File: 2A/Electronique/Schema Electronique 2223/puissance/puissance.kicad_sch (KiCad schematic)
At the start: 45 parts, among them J1 Conn_01x02, J10 Conn_01x02, J11 Conn_01x02, J12 Conn_01x02, J13 Conn_01x02, J14 Conn_01x03, J15 Conn_01x04, J16 Conn_02x20_Counter_Clockwise, J17 Connecteur bouton Arret Urgen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, J18 Bat 2, J19 Bat 1, J2 Conn_01x02, J3 Conn_01x02, J4 Conn_01x02, J5 Conn_01x02, J6 Conn_01x02, J7 Conn_01x02, J8 Conn_01x02, J9 Conn_01x02

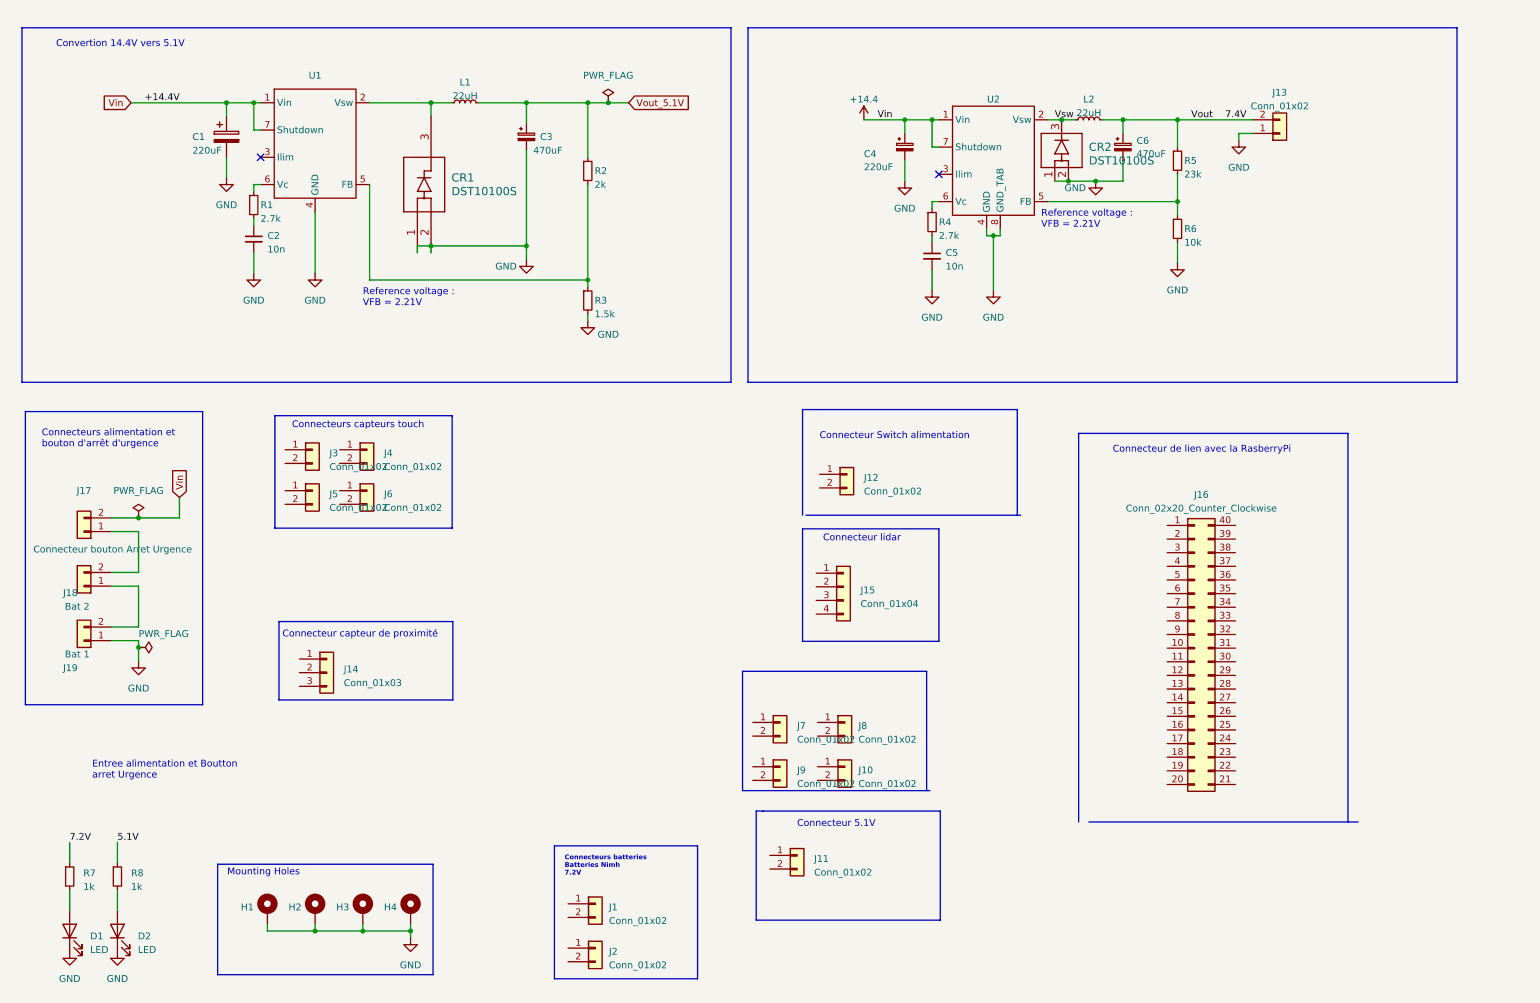
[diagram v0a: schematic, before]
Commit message: update pcb
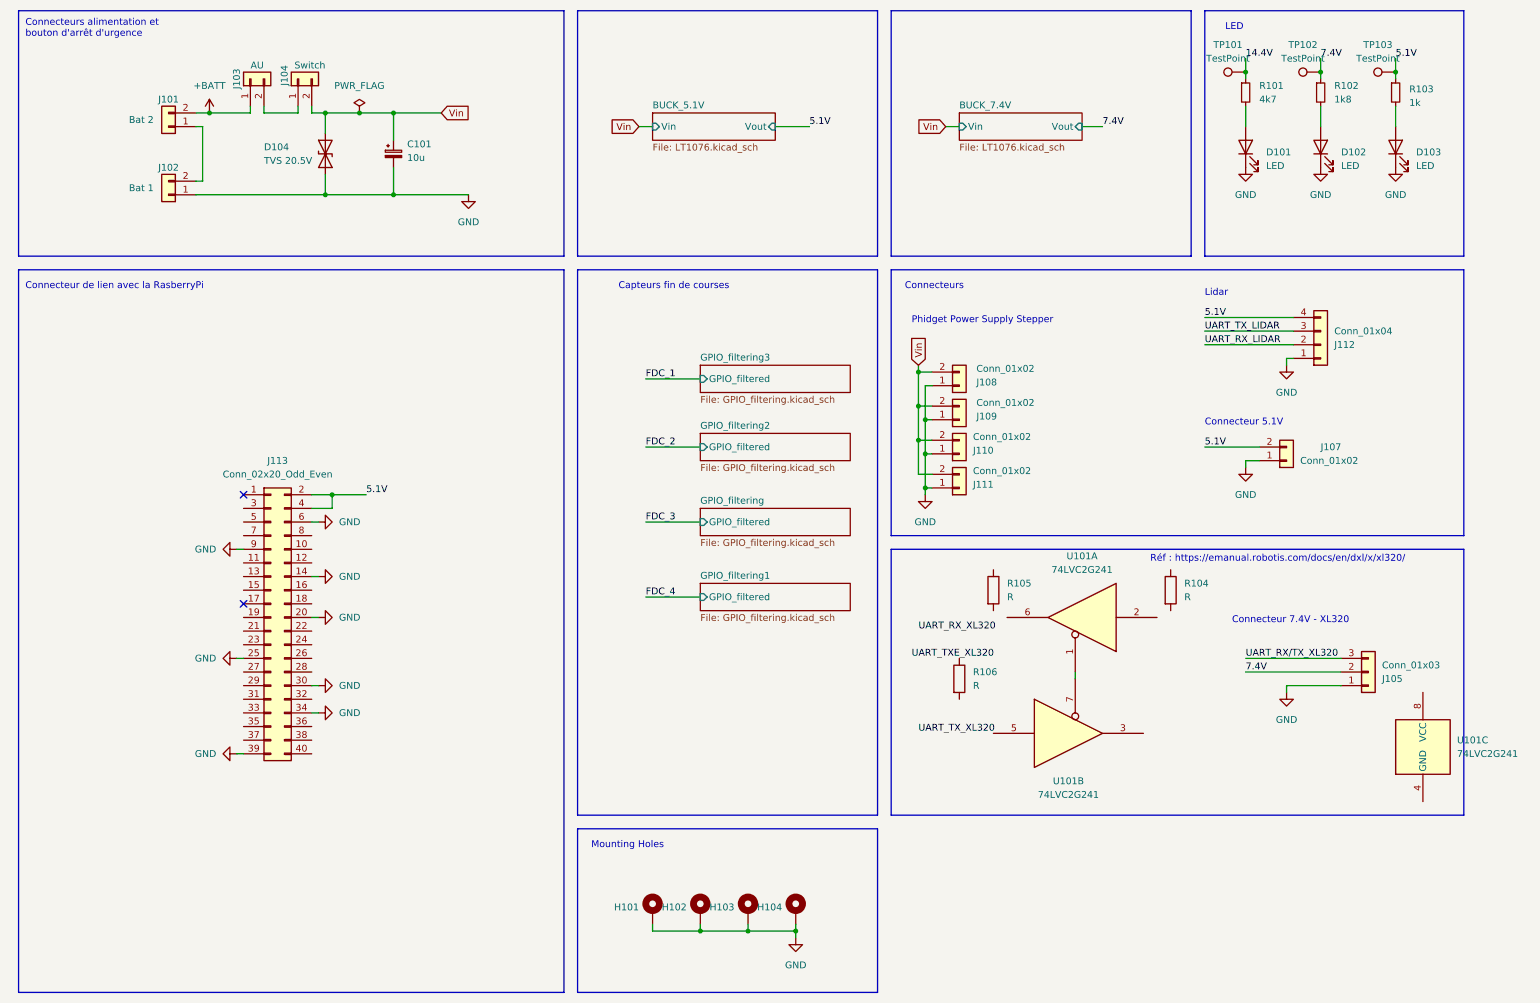
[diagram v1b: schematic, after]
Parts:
- removed C1: 220uF, Capacitor_SMD:C_0603_1608Metric_Pad1.08x0.95mm_HandSolder, symbol Device:C_Polarized
- removed C2, C5: 10n, Capacitor_SMD:C_0603_1608Metric_Pad1.08x0.95mm_HandSolder, symbol Device:C_Small
- removed C3, C6: 470uF, Capacitor_SMD:CP_Elec_10x10.5, symbol Device:C_Polarized_Small
- removed C4: 220uF, Capacitor_SMD:CP_Elec_10x10.5, symbol Device:C_Polarized_Small
- removed CR1: DST10100S, TO277B_LTF, symbol custom:DST10100S
- removed CR2: DST10100S, libs:DST10100S, symbol 2023-03-19_11-33-54:DST10100S
- removed J1, J11, J12, J2, J3, J4, J5, J6: Conn_01x02, symbol Connector_Generic:Conn_01x02
- removed J13: Conn_01x02, Connector_JST:JST_XH_B2B-XH-A_1x02_P2.50mm_Vertical, symbol Connector_Generic:Conn_01x02
- removed J14: Conn_01x03, symbol Connector_Generic:Conn_01x03
- removed J16: Conn_02x20_Counter_Clockwise, symbol Connector_Generic:Conn_02x20_Counter_Clockwise
- removed L1, L2: 22uH, Inductor_SMD:L_Wuerth_WE-PD-Typ-LS_Handsoldering, symbol Device:L_Small
- removed R1, R4: 2.7k, Resistor_SMD:R_0603_1608Metric_Pad0.98x0.95mm_HandSolder, symbol Device:R_Small
- removed R2: 2k, Resistor_SMD:R_0603_1608Metric_Pad0.98x0.95mm_HandSolder, symbol Device:R_Small
- removed R3: 1.5k, Resistor_SMD:R_0603_1608Metric_Pad0.98x0.95mm_HandSolder, symbol Device:R_Small
- removed R5: 23k, Resistor_SMD:R_0603_1608Metric_Pad0.98x0.95mm_HandSolder, symbol Device:R_Small
- removed R6: 10k, Resistor_SMD:R_0603_1608Metric_Pad0.98x0.95mm_HandSolder, symbol Device:R_Small
- removed U1: ~, symbol custom:LT1076
- removed U2: ~, libs:LT1076CR-PBF, symbol custom:LT1076
- added C101: 10u, Capacitor_SMD:CP_Elec_5x5.4, symbol Device:C_Polarized_Small
- added D101: LED, LED_SMD:LED_0603_1608Metric_Pad1.05x0.95mm_HandSolder, symbol Device:LED
- added D104: TVS 20.5V, symbol Diode:1.5KExxCA
- added J104: Switch, symbol Connector_Generic:Conn_01x02
- added J105: Conn_01x03, symbol Connector_Generic:Conn_01x03
- added J107: Conn_01x02, symbol Connector_Generic:Conn_01x02
- added J113: Conn_02x20_Odd_Even, symbol Connector_Generic:Conn_02x20_Odd_Even
- added R101: 4k7, Resistor_SMD:R_0603_1608Metric_Pad0.98x0.95mm_HandSolder, symbol Device:R_Small
- added R104, R105, R106: R, symbol Device:R
- added TP101, TP102, TP103: TestPoint, symbol Connector:TestPoint
- added U101: 74LVC2G241, symbol 74xGxx:74LVC2G241
- J103: renamed from J17; value Connecteur bouton Arret Urgence -> AU
- R102: renamed from R7; value 1k -> 1k8
- renumbered D1 to D102, D2 to D103, H1 to H101, H2 to H102, H3 to H103, H4 to H104, J18 to J101, J19 to J102, J9 to J108, J7 to J109, J8 to J110, J10 to J111, J15 to J112, R8 to R103
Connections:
- net 7.2V is gone; now on net 7.4V: R102.1
- net 5.1V: now also J112.4 (Pin_4), J107.2 (Pin_2), J113.2 (Pin_2), J113.4 (Pin_4), TP103.1
- net 7.4V: now also J105.2 (Pin_2), TP102.1
- net GND: now also J108.1 (Pin_1), J109.1 (Pin_1), J110.1 (Pin_1), J111.1 (Pin_1), J112.1 (Pin_1), C101.2, D101.1 (K), D104.2 (A2), J105.1 (Pin_1), J107.1 (Pin_1), J113.14 (Pin_14), J113.20 (Pin_20), J113.25 (Pin_25), J113.30 (Pin_30), J113.34 (Pin_34), J113.39 (Pin_39), J113.6 (Pin_6), J113.9 (Pin_9)
- net Vin: now reaches J109.2 (Pin_2)
- net Vin: now also J108.2 (Pin_2), J110.2 (Pin_2), J111.2 (Pin_2), C101.1, D104.1 (A1), J104.2 (Pin_2)
- net UART_RX_LIDAR: now reaches J112.2 (Pin_2)
- net UART_TX_LIDAR: now reaches J112.3 (Pin_3)
- net +BATT: now reaches J101.2 (Pin_2), J103.1 (Pin_1)
- net +24V: no longer names the net of J103.2 (Pin_2)
- net +24V: now also J104.1 (Pin_1)
- new net: U101.1, U101.7
- new net: D101.2 (A), R101.2
- new net 14.4V: R101.1, TP101.1
- new net UART_RX/TX_XL320: J105.3 (Pin_3)
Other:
- added sheet BUCK_5.1V (LT1076.kicad_sch)
- added sheet BUCK_7.4V (LT1076.kicad_sch)
- added sheet GPIO_filtering (GPIO_filtering.kicad_sch)
- added sheet GPIO_filtering1 (GPIO_filtering.kicad_sch)
- added sheet GPIO_filtering2 (GPIO_filtering.kicad_sch)
- added sheet GPIO_filtering3 (GPIO_filtering.kicad_sch)
- note added: "Capteurs fin de courses"
- note added: "Connecteur 7.4V - XL320"
- note added: "Connecteurs"
- note added: "LED"
- note added: "Lidar"
- note added: "Phidget Power Supply Stepper"
- note added: "Réf : https://emanual.robotis.com/docs/en/dxl/x/xl320/"
- note removed: "Connecteur Switch alimentation"
- note removed: "Connecteur capteur de proximité"
- note removed: "Connecteur lidar"
- note removed: "Connecteurs batteries Batteries Nimh 7.2V"
- note removed: "Connecteurs capteurs touch"
- note removed: "Convertion 14.4V vers 5.1V"
- note removed: "Entree alimentation et Boutton arret Urgence"
- note removed: "Reference voltage : VFB = 2.21V"
- moved on the sheet: D102, D103, H101, H102, H103, H104, J101, J102, J103, J108, J109, J110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
